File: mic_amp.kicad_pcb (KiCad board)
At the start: 2 copper layers, 33.6 x 51 mm, 39 parts

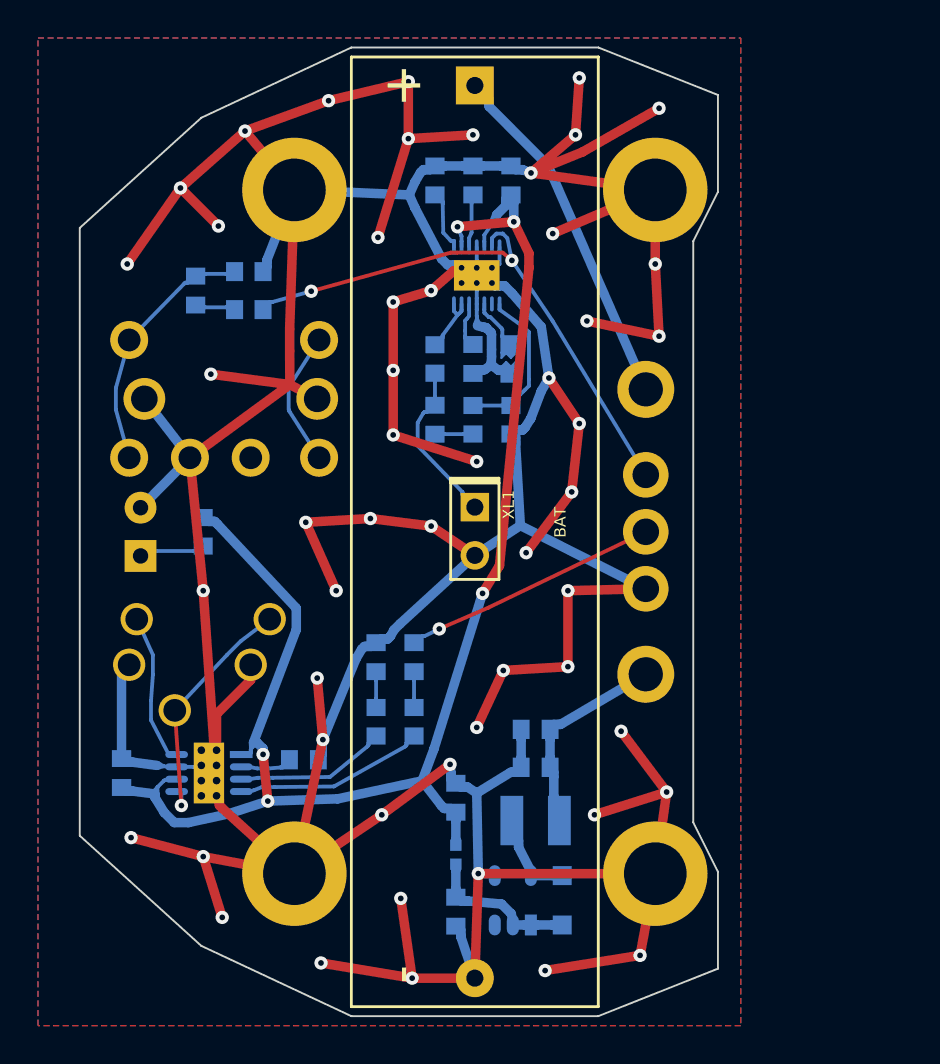
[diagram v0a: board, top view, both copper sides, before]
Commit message: + mic amp 2.1 pcb ready
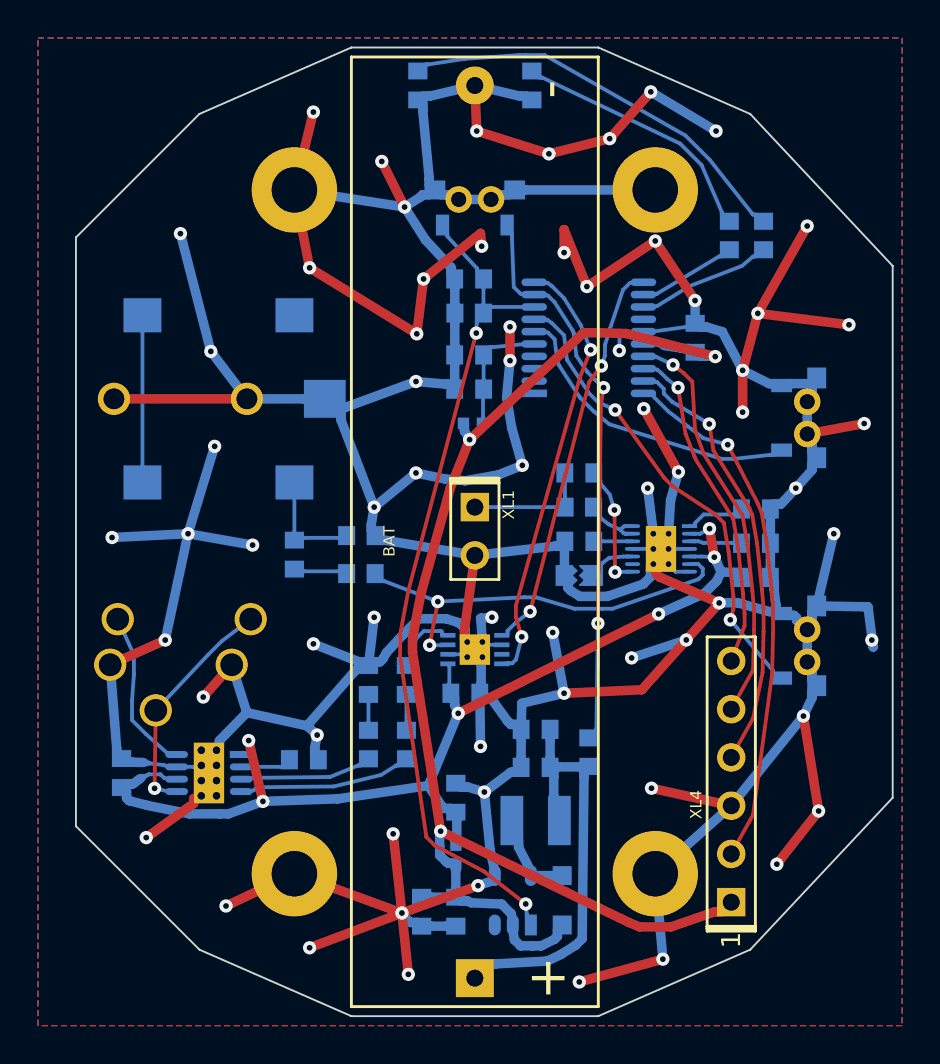
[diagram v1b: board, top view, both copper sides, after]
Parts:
- added C15: 10n, Capacitors:CAP_0603, B.Cu at (138.2, 80.6)
- added C16: 1u, Capacitors:CAP_0603, B.Cu at (138.2, 82.4)
- added C17: 0.1u, Capacitors:CAP_0603, B.Cu at (150.1, 79.7)
- added C18: 0.1u, Capacitors:CAP_0603, B.Cu at (138.0, 98.4)
- added C19: 10u, Capacitors:CAP_0603, B.Cu at (138.2, 76.6)
- added C20: 0.1u, Capacitors:CAP_0603, B.Cu at (135.7, 109.9)
- added D4: LED, LEDs:LED_0603, B.Cu at (135.5, 66.4)
- added DD1: STM32F030F6Px, SO_DIL_TSSOP:TSSOP20, B.Cu at (144.5, 79.7)
- added DD2: MC4011, QFN_DFN:DFN8_2x3, B.Cu at (138.5, 96.1)
- added L3: BLM15AG102, Inductors:IND_0402, B.Cu at (138.4, 84.2)
- added SW1: IT-1198E, BtnsSwitches:BTN_IT1198, B.Cu at (156.0, 83.9)
- added SW2: IT-1198E, BtnsSwitches:BTN_IT1198, B.Cu at (156.0, 95.9)
- added SW3: IT-1198E, BtnsSwitches:BTN_IT1198, B.Cu at (138.5, 72.4)
- added XL4: CONN_6, Connectors:PLS-6, F.Cu at (152.0, 109.4)
- D1: footprint LEDs:LED_Through-Hole-3mm -> LEDs:LED_0603
- D3: value BAT54WS -> PMEG3010
- HOLE1, HOLE2, HOLE3, HOLE4: footprint PCB:Hole3d3_out5d5mm -> PCB:Hole2d4_out4d5mm
- R2: value 0R -> 10k
- R3: value DNM -> 390k
- R4: value 2k -> 1k
- R5: value RVarWSw -> 1k; footprint Resistors:RVar_SP3_R -> Resistors:RES_0603
- R8: value 0R -> 15k
- XL3: footprint Connectors:Audio_ST013 -> Connectors:Audio_ST511D01TR
- moved R4 31.8 mm to (151.9, 74.3), turned to 90 degrees
- moved D1 31.3 mm to (141.5, 66.4), turned to 270 degrees
- moved C5 24.6 mm to (153.3, 92.3), turned to 0 degrees
- moved C4 24.2 mm to (153.3, 90.5), turned to 0 degrees
- moved C3 24.2 mm to (153.3, 88.7), turned to 0 degrees
- moved R2 18.5 mm to (144.5, 101.5)
- moved D2 17.4 mm to (148.3, 90.8), turned to 270 degrees
- moved R5 16.1 mm to (153.7, 74.3)
- moved R8 15.1 mm to (132.5, 92.1)
- moved R9 15.1 mm to (132.5, 90.1)
- moved C9 14.8 mm to (129.0, 91.1)
- moved F1 12.0 mm to (144.0, 92.2), turned to 180 degrees
- moved C2 11.1 mm to (144.0, 90.4), turned to 180 degrees
- moved R1 10.9 mm to (144.0, 88.6), turned to 0 degrees
- moved C1 8.10 mm to (144.0, 86.8), turned to 0 degrees
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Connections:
- B1 pad A: /BAT_IN -> +BATT
- C1 pad 2: Net-(C1-Pad2) -> /MICIN
- C6 pad 1: Net-(C6-Pad1) -> /W
- D2 pad 6: /Output -> /MicAmpOut
- DA2 pad 1: /3v3unfil -> /PWR_EN
- R2 pad 1: Net-(C1-Pad2) -> +BATT
- R2 pad 2: /MICIN -> /BTN_CHCK
- R3 pad 1: /MICIN -> /PWR_EN
- R4 pad 1: +3.3V -> Net-(DD1-Pad12)
- R5 pad 1: /Output -> Net-(DD1-Pad13)
- R5 pad 2: GND -> Net-(D4-PadA)
- R8 pad 2: /Output -> /MicAmpOut
- XL3 pad 2: (no net) -> Net-(XL3-Pad2)
- XL3 pad 3: Net-(XL3-Pad3) -> (no net)
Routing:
- net /3v3unfil: track 8.14 -> 72.5 mm, vias 0 -> 3
- net GND: track 366.1 -> 428.0 mm, vias 52 -> 67
- net /PWR_EN: track 0.00 -> 44.1 mm, vias 0 -> 2
- net /Output: track 29.8 -> 0.00 mm, vias 2 -> 0
- net /BTN_CHCK: track 0.00 -> 29.7 mm, vias 0 -> 2
- net /SWCLK: track 0.00 -> 27.8 mm, vias 0 -> 1
- net +3.3V: track 83.0 -> 57.8 mm, vias 5 -> 6
- net Net-(DD1-Pad7): track 0.00 -> 24.6 mm, vias 0 -> 2
- net /SWDIO: track 0.00 -> 22.9 mm, vias 0 -> 1
- net /UD: track 0.00 -> 22.7 mm, vias 0 -> 2
- net /MicAmpOut: track 0.00 -> 22.5 mm, vias 0 -> 2
- net Net-(D4-PadA): track 0.00 -> 21.5 mm
- net /UART_TX: track 0.00 -> 21.3 mm, vias 0 -> 1
- net /CS: track 0.00 -> 21.0 mm, vias 0 -> 2
- net /BAT_IN: track 18.7 -> 0.00 mm
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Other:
- board size 33.6 x 51 mm -> 43 x 51 mm
- net class Default: via_dia 0.8 -> 0.7
- net class wide: via_dia 0.8 -> 0.7
- board text added: "-"
- board text added: "Mic Amp"
- board text added: "MicAmp v4"
- board text added: "Power"
